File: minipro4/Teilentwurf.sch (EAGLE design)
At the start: 62 parts, among them IC1 MEGA8-P, IC2 FT232RL_ADAPTER, IC3 78L08Z, IC4 4051N, J1 HOHLSTECKER, Q2 BS170, Q3 BS170, Q4 BS170, Q6 IRF4905, X1 , X2 CON_COAX

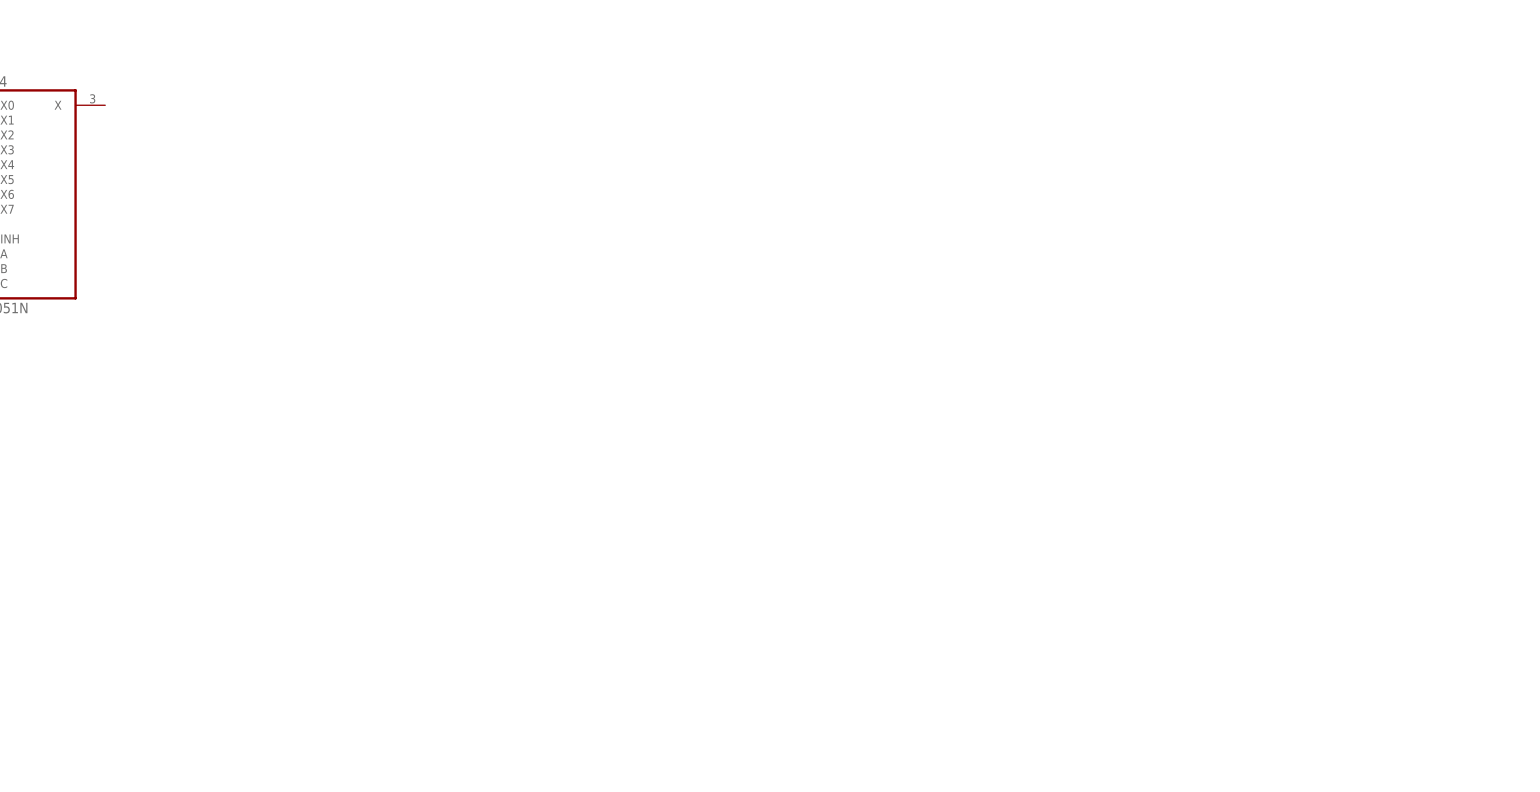
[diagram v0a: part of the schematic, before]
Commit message: < ‘minipro4/Teilentwurf.b##’ > ‘minipro4/Teilentwurf.b#1’ / ‘minipro4/Teilentwurf.brd’ < ‘minipro4/Teilentwurf.s##’ > ‘minipro4/Teilentwurf.s#1’ / ‘minipro4/Teilentwurf.sch’
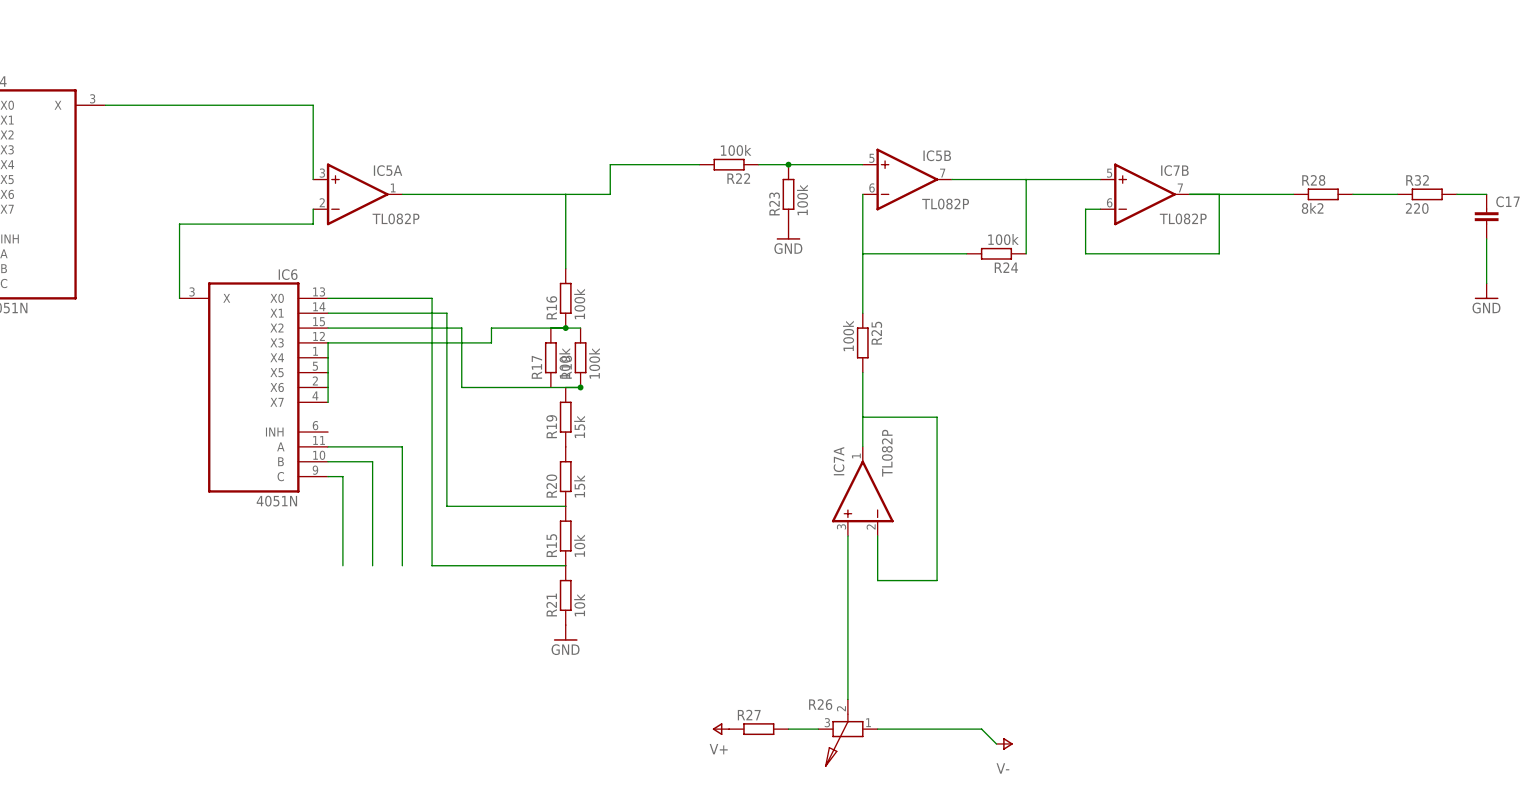
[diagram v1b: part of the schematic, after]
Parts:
- added C17: (no value), 03_device-library:C-EU025-030X050
- added IC5, IC7: TL082P, 03_device-library:TL082P
- added IC6: 4051N, 03_device-library:4051N
- added R15, R21: 10k, 03_device-library:R-EU_0207/10
- added R16, R17, R18, R22, R23, R24, R25: 100k, 03_device-library:R-EU_0207/10
- added R19, R20: 15k, 03_device-library:R-EU_0207/10
- added R26: (no value), 03_device-library:POT
- added R27: (no value), 03_device-library:R-EU_0207/10
- added R28: 8k2, 03_device-library:R-EU_0207/10
- added R32: 220, 03_device-library:R-EU_0207/10
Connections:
- new net N$25: IC4A.X, IC5A.+IN
- new net N$26: IC5A.-IN, IC6A.X
- new net N$27: IC5B.+IN, R22.1, R23.2
- new net N$28: R19.1, R20.2
- new net N$31: IC6A.X0, R15.1, R21.2
- new net N$32: IC6A.X1, R15.2, R20.1
- new net N$33: IC6A.X2, R17.1, R18.1, R19.2
- new net N$34: IC5A.OUT, R16.2, R22.2
- new net N$35: IC5B.OUT, IC7B.+IN, R24.1
- new net N$36: IC5B.-IN, R24.2, R25.1
- new net N$37: IC7A.-IN, IC7A.OUT, R25.2
- new net N$38: R26.2, R27.2
- new net N$39: IC7A.+IN, R26.3
- new net N$40: IC7B.-IN, IC7B.OUT, R28.1
- new net N$41: R28.2, R32.1
- new net N$42: C17.1, R32.2
- net GND: now also C17.2, R21.1, R23.1
- net MUX0*: now also IC6A.A, IC6A.X3, IC6A.X4, IC6A.X5, IC6A.X6, IC6A.X7, R16.1, R17.2, R18.2
- net MUX1*: now also IC6A.B
- net MUX2*: now also IC6A.C
- net V+: now also R27.1
- net V-: now also R26.1

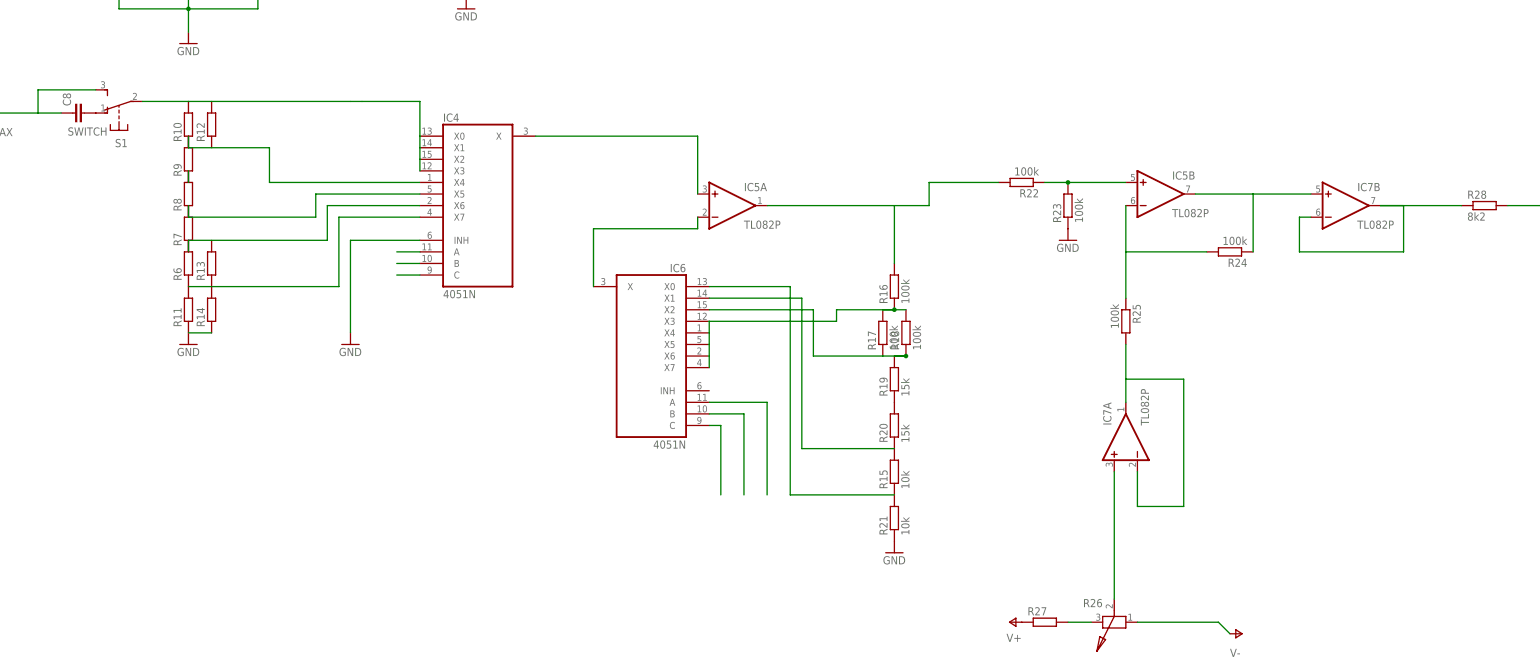
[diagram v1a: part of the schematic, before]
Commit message: / ‘minipro4/Teilentwurf.b#1’ < ‘minipro4/Teilentwurf.b##’ > ‘minipro4/Teilentwurf.b#2’ / ‘minipro4/Teilentwurf.brd’ / ‘minipro4/Teilentwurf.s#1’ < ‘minipro4/Teilentwurf.s##’ > ‘minipro4/Teilentwurf.s#2’ / ‘minipro4/Teilentwurf.sch’
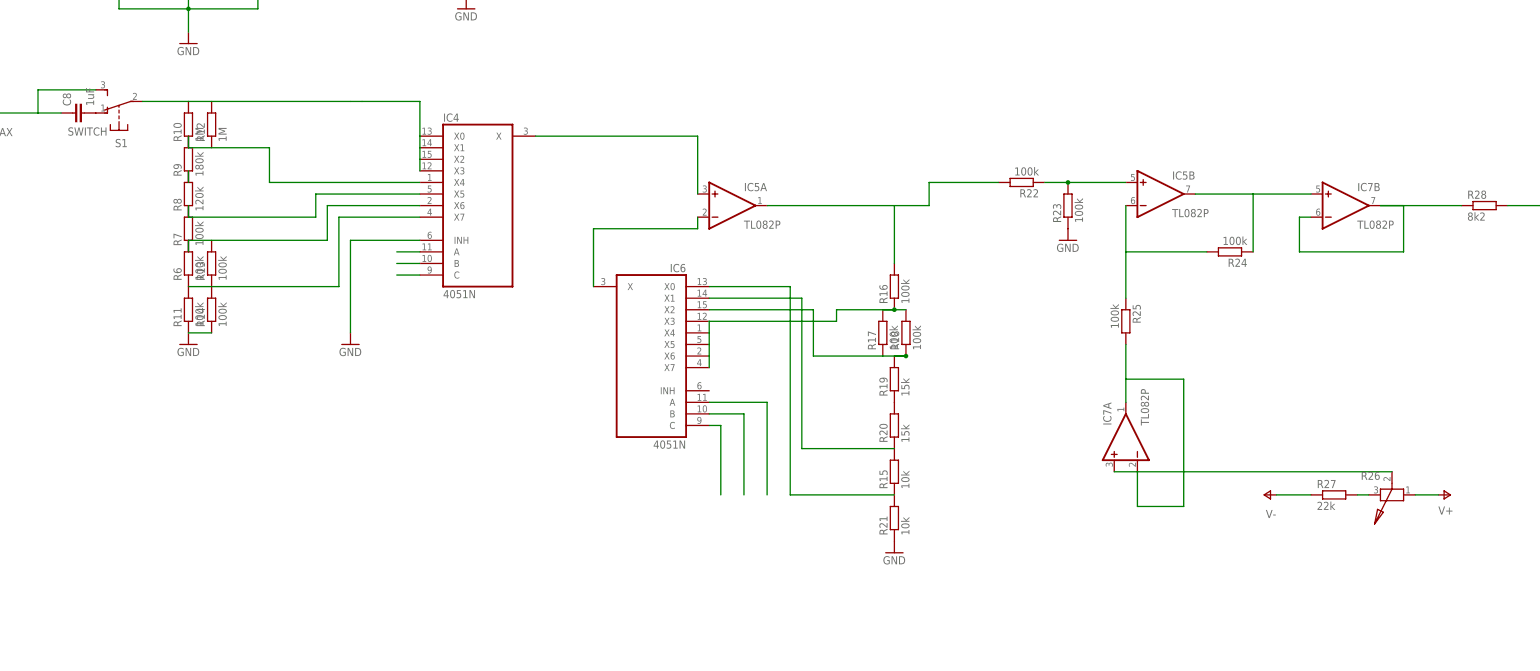
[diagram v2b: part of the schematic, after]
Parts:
- C8: value (none) -> 1uF
- R10, R12: value (none) -> 1M
- R11, R13, R14, R6, R7: value (none) -> 100k
- R27: value (none) -> 22k
- R8: value (none) -> 120k
- R9: value (none) -> 180k
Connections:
- net V+: now also R26.1; no longer R27.1
- net V-: now also R27.1; no longer R26.1
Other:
- moved on the sheet: R26, R27
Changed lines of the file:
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@@
 <part name="GND11" library="03_device-library" deviceset="GND" device=""/>
 <part name="FRAME1" library="frames" deviceset="DINA4_L" device="" value="Vorgabe"/>
-<part name="R6" library="03_device-library" deviceset="R-EU_" device="0207/10"/>
-<part name="R7" library="03_device-library" deviceset="R-EU_" device="0207/10"/>
-<part name="R8" library="03_device-library" deviceset="R-EU_" device="0207/10"/>
-<part name="R9" library="03_device-library" deviceset="R-EU_" device="0207/10"/>
-<part name="R10" library="03_device-library" deviceset="R-EU_" device="0207/10"/>
-<part name="R11" library="03_device-library" deviceset="R-EU_" device="0207/10"/>
-<part name="R12" library="03_device-library" deviceset="R-EU_" device="0207/10"/>
-<part name="R13" library="03_device-library" deviceset="R-EU_" device="0207/10"/>
-<part name="R14" library="03_device-library" deviceset="R-EU_" device="0207/10"/>
+<part name="R6" library="03_device-library" deviceset="R-EU_" device="0207/10" value="100k"/>
+<part name="R7" library="03_device-library" deviceset="R-EU_" device="0207/10" value="100k"/>
+<part name="R8" library="03_device-library" deviceset="R-EU_" device="0207/10" value="120k"/>
+<part name="R9" library="03_device-library" deviceset="R-EU_" device="0207/10" value="180k"/>
+<part name="R10" library="03_device-library" deviceset="R-EU_" device="0207/10" value="1M"/>
+<part name="R11" library="03_device-library" deviceset="R-EU_" device="0207/10" value="100k"/>
+<part name="R12" library="03_device-library" deviceset="R-EU_" device="0207/10" value="1M"/>
+<part name="R13" library="03_device-library" deviceset="R-EU_" device="0207/10" value="100k"/>
+<part name="R14" library="03_device-library" deviceset="R-EU_" device="0207/10" value="100k"/>
 <part name="GND9" library="03_device-library" deviceset="GND" device=""/>
 <part name="IC4" library="03_device-library" deviceset="4051" device="N"/>
 <part name="S1" library="03_device-library" deviceset="SWITCH" device=""/>
-<part name="C8" library="03_device-library" deviceset="C-EU" device="050-050X075"/>
+<part name="C8" library="03_device-library" deviceset="C-EU" device="050-050X075" value="1uF"/>
 <part name="X2" library="03_device-library" deviceset="CON_COAX" device=""/>
 <part name="GND12" library="03_device-library" deviceset="GND" device=""/>
@@
 <part name="P-2" library="03_device-library" deviceset="V-" device=""/>
 <part name="R26" library="03_device-library" deviceset="POT" device=""/>
-<part name="R27" library="03_device-library" deviceset="R-EU_" device="0207/10"/>
+<part name="R27" library="03_device-library" deviceset="R-EU_" device="0207/10" value="22k"/>
 <part name="R28" library="03_device-library" deviceset="R-EU_" device="0207/10" value="8k2"/>
 <part name="R32" library="03_device-library" deviceset="R-EU_" device="0207/10" value="220"/>
@@
 <instance part="IC7" gate="B" x="297.18" y="-30.48"/>
 <instance part="R25" gate="G$1" x="248.92" y="-55.88" rot="R270"/>
-<instance part="P+4" gate="1" x="223.52" y="-121.92" rot="R90"/>
-<instance part="P-2" gate="1" x="274.32" y="-124.46" rot="R90"/>
-<instance part="R26" gate="G$1" x="246.38" y="-121.92" rot="R180"/>
-<instance part="R27" gate="G$1" x="231.14" y="-121.92"/>
+<instance part="P+4" gate="1" x="320.04" y="-93.98" rot="MR90"/>
+<instance part="P-2" gate="1" x="279.4" y="-93.98" rot="MR90"/>
+<instance part="R26" gate="G$1" x="307.34" y="-93.98" rot="R180"/>
+<instance part="R27" gate="G$1" x="294.64" y="-93.98"/>
 <instance part="R28" gate="G$1" x="327.66" y="-30.48"/>
 <instance part="R32" gate="G$1" x="345.44" y="-30.48"/>
@@
 </segment>
 <segment>
+<pinref part="R26" gate="G$1" pin="1"/>
 <pinref part="P+4" gate="1" pin="V+"/>
-<pinref part="R27" gate="G$1" pin="1"/>
+<wire x1="317.5" y1="-93.98" x2="312.42" y2="-93.98" width="0.1524" layer="91"/>
 </segment>
 </net>
@@
 </segment>
 <segment>
-<pinref part="R26" gate="G$1" pin="1"/>
+<pinref part="R27" gate="G$1" pin="1"/>
 <pinref part="P-2" gate="1" pin="V-"/>
-<wire x1="251.46" y1="-121.92" x2="269.24" y2="-121.92" width="0.1524" layer="91"/>
-<wire x1="269.24" y1="-121.92" x2="271.78" y2="-124.46" width="0.1524" layer="91"/>
+<wire x1="281.94" y1="-93.98" x2="289.56" y2="-93.98" width="0.1524" layer="91"/>
 </segment>
 </net>
@@
 <pinref part="R27" gate="G$1" pin="2"/>
 <pinref part="R26" gate="G$1" pin="2"/>
-<wire x1="236.22" y1="-121.92" x2="241.3" y2="-121.92" width="0.1524" layer="91"/>
+<wire x1="299.72" y1="-93.98" x2="302.26" y2="-93.98" width="0.1524" layer="91"/>
 </segment>
 </net>
@@
 <pinref part="R26" gate="G$1" pin="3"/>
 <pinref part="IC7" gate="A" pin="+IN"/>
-<wire x1="246.38" y1="-116.84" x2="246.38" y2="-88.9" width="0.1524" layer="91"/>
-</segment>
-</net>
+<wire x1="307.34" y1="-88.9" x2="246.38" y2="-88.9" width="0.1524" layer="91"/>
+</segment>
+</net>
